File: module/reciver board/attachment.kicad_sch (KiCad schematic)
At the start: 8 parts, among them U13 OSMC Module Board, U14 OSMC Module Board, U15 OSMC Module Board, U16 OSMC Module Board, U17 OSMC Module Board, U18 OSMC Module Board, U19 OSMC Module Board, U20 OSMC Module Board

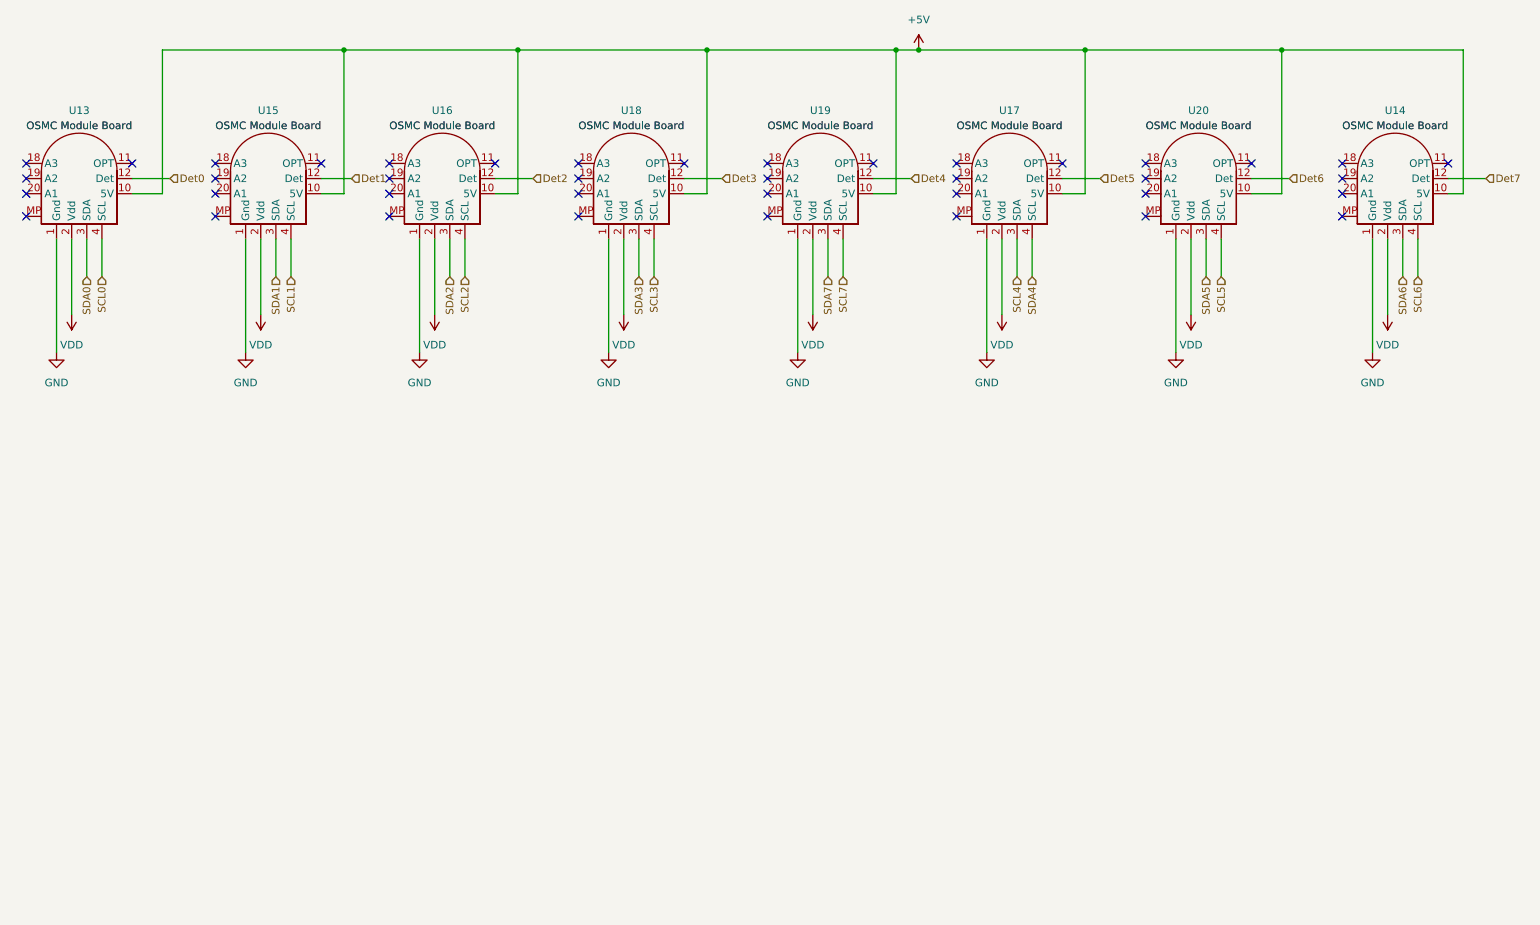
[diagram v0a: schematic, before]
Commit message: started routing
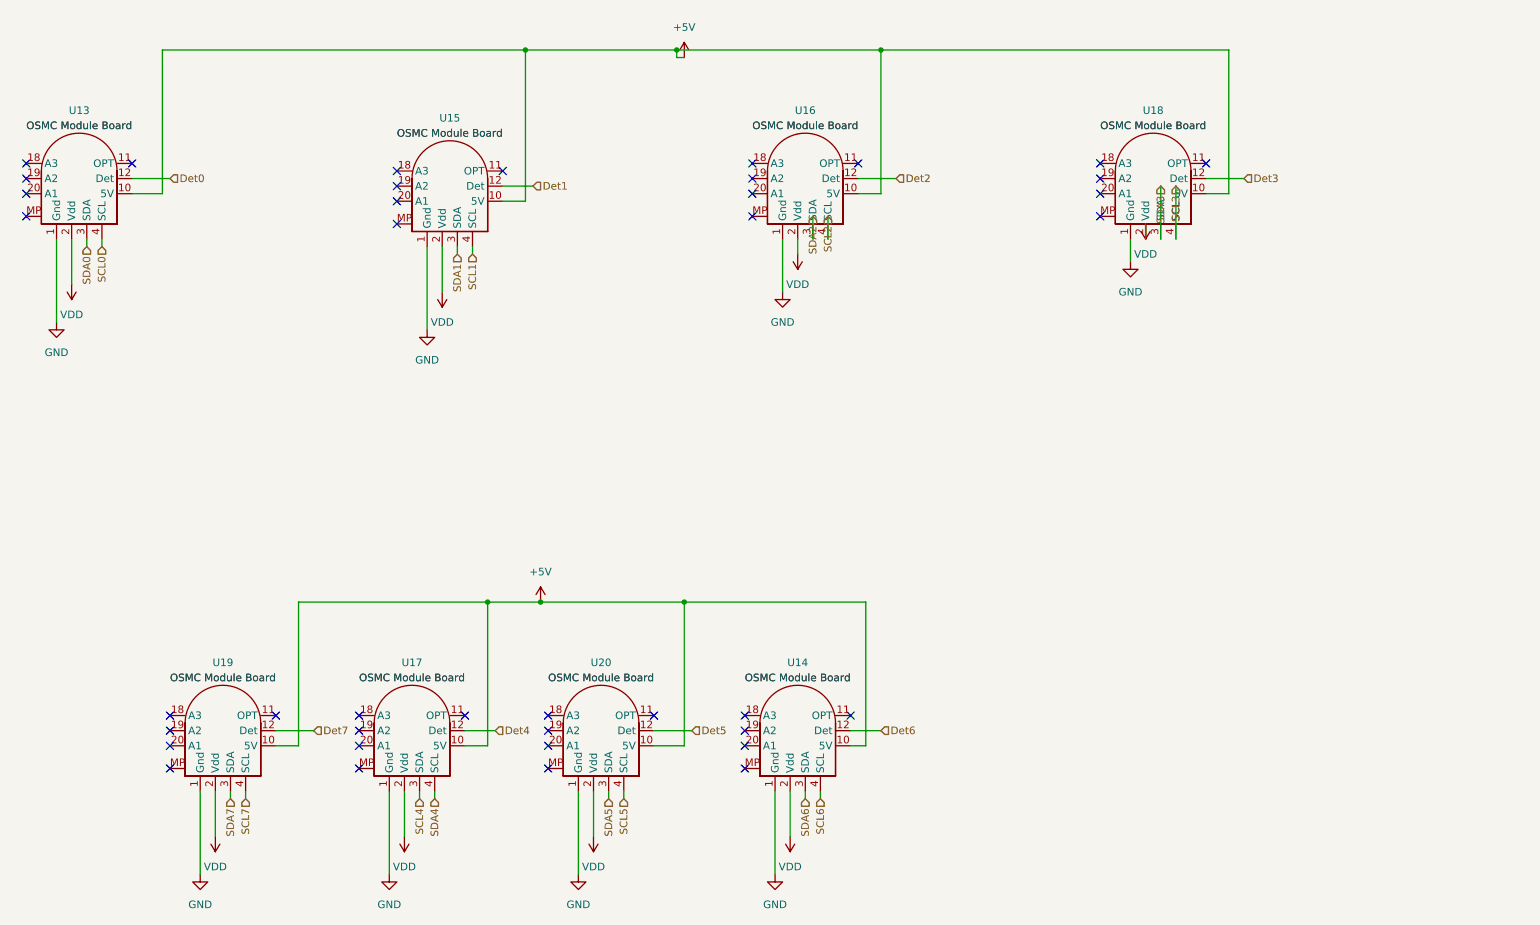
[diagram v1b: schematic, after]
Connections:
- net Det4: now also U17.12 (Det), U17.13 (Det); no longer U19.12 (Det), U19.13 (Det)
- net Det5: now also U20.12 (Det), U20.13 (Det); no longer U17.12 (Det), U17.13 (Det)
- net Det6: now also U14.12 (Det), U14.13 (Det); no longer U20.12 (Det), U20.13 (Det)
- net Det7: now also U19.12 (Det), U19.13 (Det); no longer U14.12 (Det), U14.13 (Det)
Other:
- moved on the sheet: U14, U15, U16, U17, U18, U19, U20
